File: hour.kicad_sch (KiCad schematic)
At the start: 15 parts, among them SW3 SW_MEC_5G, SW4 SW_MEC_5G, U10 4081, U11 4510, U6 4071, U9 4510

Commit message: finishing the footprint asigment
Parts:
- C13, C14, C15, C16, C17: footprint (none) -> Resistor_SMD:R_0603_1608Metric; LCSC Part (none) -> C1591
- R10, R8: footprint (none) -> Resistor_SMD:R_0603_1608Metric; LCSC Part (none) -> C14675
- R7, R9: footprint (none) -> Resistor_SMD:R_0603_1608Metric; LCSC Part (none) -> C98220
- SW3, SW4: footprint Button_Switch_SMD:SW_MEC_5GSH9 -> Button_Switch_THT:SW_PUSH_6mm_H5mm; LCSC Part (none) -> C42416244
- U10: footprint Package_DIP:DIP-14_W7.62mm_Socket_LongPads -> Package_SO:SOIC-14_3.9x8.7mm_P1.27mm; LCSC Part (none) -> C40551
- U11, U9: footprint (none) -> Package_SO:TSSOP-16_4.4x5mm_P0.65mm; LCSC Part (none) -> C2862976
- U6: footprint (none) -> Package_SO:SOIC-14_3.9x8.7mm_P1.27mm; LCSC Part (none) -> C97039

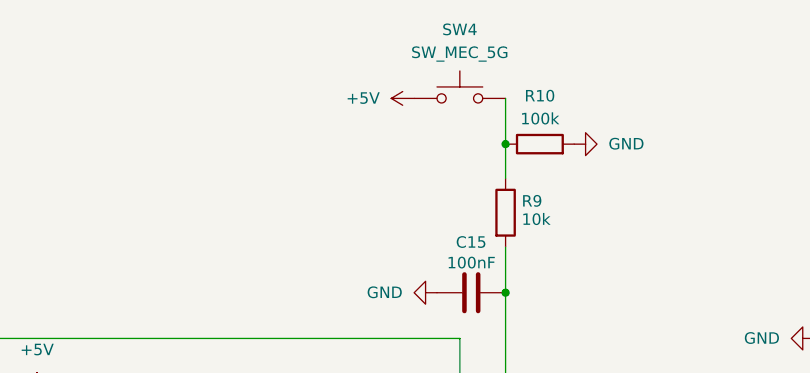
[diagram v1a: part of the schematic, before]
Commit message: starting the layout
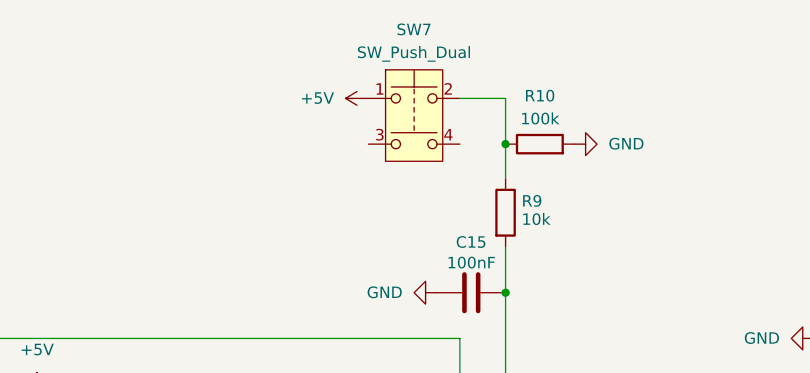
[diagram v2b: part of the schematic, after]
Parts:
- removed SW4: SW_MEC_5G, Button_Switch_THT:SW_PUSH_6mm_H5mm, symbol Switch:SW_MEC_5G
- added SW7: SW_Push_Dual, Button_Switch_THT:SW_PUSH_6mm_H5mm, symbol Switch:SW_Push_Dual
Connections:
- net +5V: now also SW7.1
- net at R10.1, R9.1: now also SW7.2
